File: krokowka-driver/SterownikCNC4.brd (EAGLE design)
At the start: 65.7 x 58.4 mm, 57 parts, among them IC1 NC7WP14P6X, IC4 NC7WP14P6X, Q1 IRF3704S, Q2 IRF3704S, Q3 IRF3704S, Q4 IRF3704S, Q5 IRF3704S, Q6 IRF3704S, Q7 IRF3704S, Q8 IRF3704S, U1 IR2104, U2 IR2104, U3 IR2104, U4 IR2104

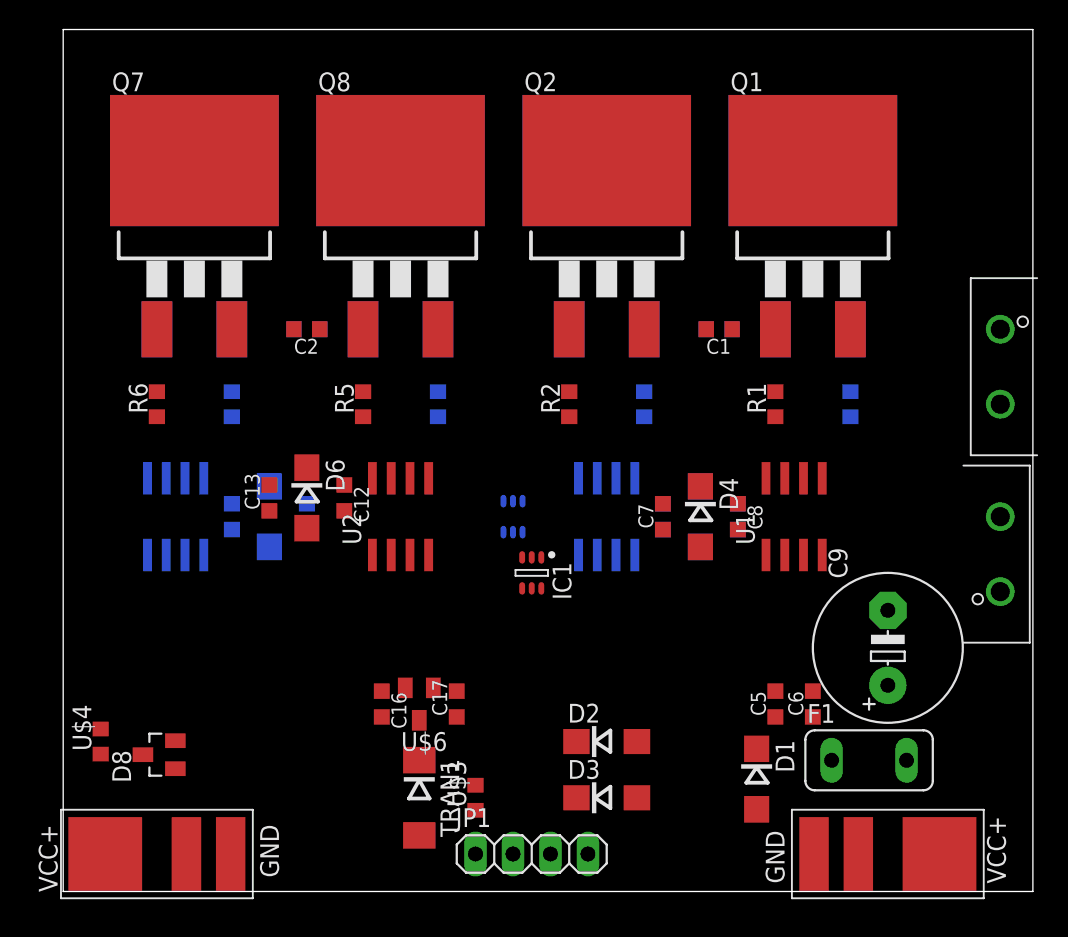
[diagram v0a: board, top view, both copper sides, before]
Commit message: zmina_30.12
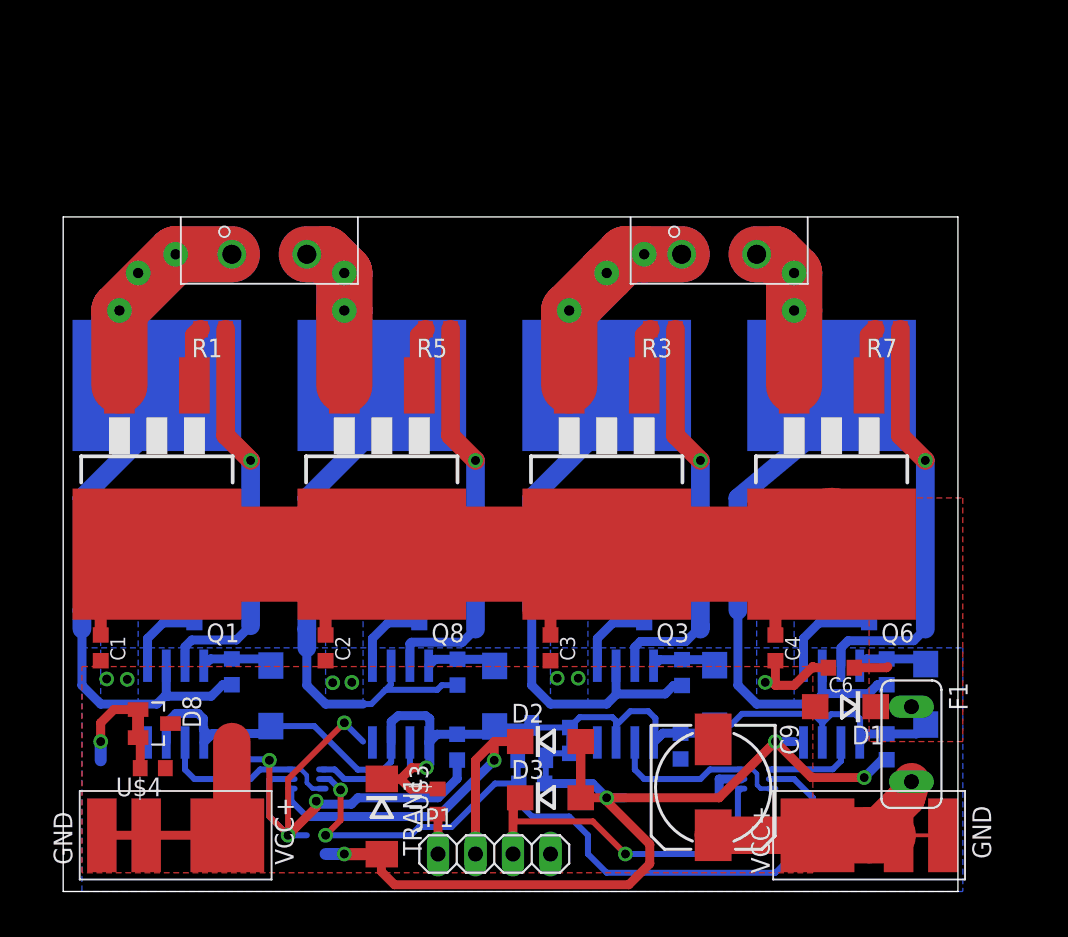
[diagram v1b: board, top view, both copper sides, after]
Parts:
- removed C5: 1uF/50v, rcl:C0603K
- C9: value 100uF/63V -> 100uF; device rcl:E5-10,5 -> rcl:153CLV-0810
- moved U$7 50.1 mm to (14.0, 43.2), turned to 0 degrees
- moved Q1 49.4 mm to (6.35, 25.4), turned to 180 degrees
- moved C1 47.1 mm to (2.54, 16.5), turned to 270 degrees
- moved U1 43.8 mm to (7.62, 12.7), flipped to the bottom
- moved R1 38.4 mm to (10.2, 38.1), turned to 180 degrees
- moved C4 38.4 mm to (48.3, 16.5), flipped to the top, turned to 270 degrees
- moved C8 35.9 mm to (11.4, 14.9), flipped to the bottom
- moved Q3 35.3 mm to (36.8, 25.4), flipped to the top, turned to 180 degrees
- moved Q2 34.1 mm to (6.35, 31.8), flipped to the bottom
- moved U3 33.0 mm to (38.1, 12.7)
- moved C7 33.0 mm to (11.6, 9.83), flipped to the bottom, turned to 270 degrees
- moved D5 32.5 mm to (44.1, 13.3)
- moved C10 32.3 mm to (41.9, 14.8)
- moved D4 31.5 mm to (14.1, 13.3), flipped to the bottom
- moved C11 29.7 mm to (41.8, 9.86), turned to 270 degrees
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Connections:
- removed net +12V: C11.1, C13.1, C14.1, C7.1, D4.A, D5.A, D6.A, D7.A, U1.1, U2.1, U3.1, U4.1
- net +24V: no longer C5.1, C9.+
- net GNDA: no longer C5.2
- net N$13: now also C9.+
- net VCC: now also C11.1, C13.1, C14.1, C7.1, D4.A, D5.A, D6.A, D7.A, U1.1, U2.1, U3.1, U4.1
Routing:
- net GND: track 0.00 -> 126.7 mm, vias 0 -> 9
- net VCC: track 0.00 -> 83.5 mm, vias 0 -> 1
- net +24V: track 0.00 -> 76.4 mm
- net M_OUT: track 0.00 -> 68.4 mm, vias 0 -> 2
- net M_OUT2: track 0.00 -> 66.5 mm, vias 0 -> 3
- net M_OUT3: track 0.00 -> 60.0 mm, vias 0 -> 2
- net M_OUT1: track 0.00 -> 59.2 mm, vias 0 -> 2
- net +3V3: track 0.00 -> 52.2 mm, vias 0 -> 2
- net N$20: track 0.00 -> 28.5 mm, vias 0 -> 1
- net PWM1: track 0.00 -> 27.8 mm, vias 0 -> 1
- net N$7: track 0.00 -> 27.4 mm, vias 0 -> 1
- net N$14: track 0.00 -> 27.3 mm, vias 0 -> 1
- net N$3: track 0.00 -> 27.1 mm, vias 0 -> 1
- net PWM2: track 0.00 -> 25.7 mm, vias 0 -> 1
- net N$13: track 0.00 -> 20.3 mm
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- added copper zone on layer 1, net +24V
- added copper zone on layer 16, net GND
- added copper zone on layer 1, net GNDA
- added copper zone on layer 16, net GNDA
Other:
- board size 65.7 x 58.4 mm -> 60.6 x 45.7 mm
- board text added: "Czy tych złącz nie da się ścisnąć?"
- board text added: "Logika i zasilanie 12v do wyplatania"
- board text added: "Napisy do poprawienia"
- board text added: "Pamietac o ERC 8mils"
- board text added: "Sprawdzić: 1. Kondensator polimerowy 2. Bezpiecznik +24V"
- board text removed: "Podmieniłem footprint kondensatora 100uF"
